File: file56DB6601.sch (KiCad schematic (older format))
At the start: 1 part, among them U2 SHT21

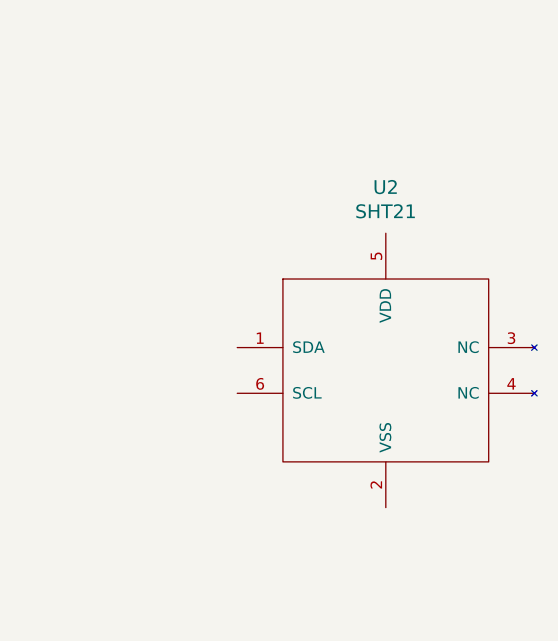
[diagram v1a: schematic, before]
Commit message: started layout, completed schematic
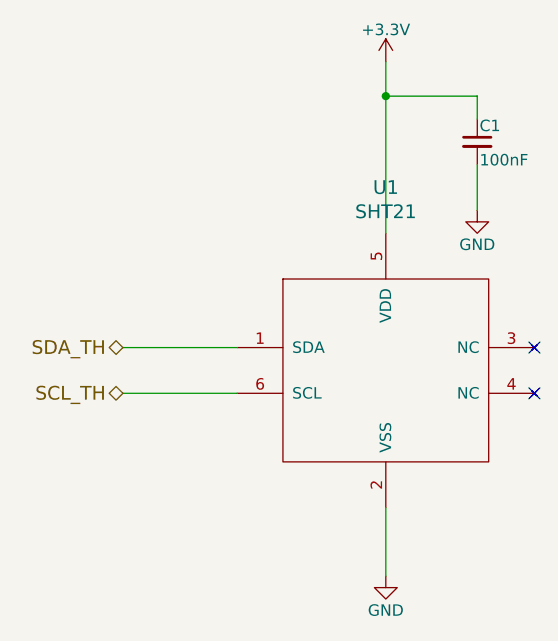
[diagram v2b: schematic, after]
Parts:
- added C1: 100nF, symbol C_Small
- renumbered U2 to U1
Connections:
- net SDA_TH: now reaches U1.1 (SDA)
- net GND: now reaches U1.2 (VSS)
- net GND: now also C1.2
- net +3V3: now reaches U1.5 (VDD)
- net +3V3: now also C1.1
- net SCL_TH: now reaches U1.6 (SCL)
- no-connect marks 0 -> 2
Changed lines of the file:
@@
 LIBS:mpu-9250
 LIBS:SAMD21E17A
+LIBS:miniultrapro
+LIBS:texas-instruments
 LIBS:lorawan_gps-cache
 EELAYER 25 0
@@
 $Descr A4 11693 8268
 encoding utf-8
-Sheet 3 7
+Sheet 2 7
 Title ""
 Date ""
@@
 $EndDescr
 $Comp
-L SHT21 U2
+L SHT21 U1
 U 1 1 56DB6717
 P 5650 3200
-F 0 "U2" H 5650 4000 60  0000 C CNN
+F 0 "U1" H 5650 4000 60  0000 C CNN
 F 1 "SHT21" H 5650 3894 60  0000 C CNN
 F 2 "timhawes:SHT21" H 5650 3200 60  0001 C CNN
@@
 	1    0    0    -1
 $EndComp
+$Comp
+L GND #PWR2
+U 1 1 56EA146B
+P 5650 4100
+F 0 "#PWR2" H 5650 3850 50  0001 C CNN
+F 1 "GND" H 5650 3950 50  0000 C CNN
+F 2 "" H 5650 4100 50  0000 C CNN
+F 3 "" H 5650 4100 50  0000 C CNN
+	1    5650 4100
+	1    0    0    -1
+$EndComp
+$Comp
+L +3.3V #PWR1
+U 1 1 56EA1481
+P 5650 1850
+F 0 "#PWR1" H 5650 1700 50  0001 C CNN
+F 1 "+3.3V" H 5650 1990 50  0000 C CNN
+F 2 "" H 5650 1850 50  0000 C CNN
+F 3 "" H 5650 1850 50  0000 C CNN
+	1    5650 1850
+	1    0    0    -1
+$EndComp
+$Comp
+L GND #PWR3
+U 1 1 56EA1497
+P 6050 2500
+F 0 "#PWR3" H 6050 2250 50  0001 C CNN
+F 1 "GND" H 6050 2350 50  0000 C CNN
+F 2 "" H 6050 2500 50  0000 C CNN
+F 3 "" H 6050 2500 50  0000 C CNN
+	1    6050 2500
+	1    0    0    -1
+$EndComp
+$Comp
+L C_Small C1
+U 1 1 56EA1572
+P 6050 2200
+F 0 "C1" H 6060 2270 50  0000 L CNN
+F 1 "100nF" H 6060 2120 50  0000 L CNN
+F 2 "" H 6050 2200 50  0000 C CNN
+F 3 "" H 6050 2200 50  0000 C CNN
+	1    6050 2200
+	1    0    0    -1
+$EndComp
+Wire Wire Line
+	5650 1850 5650 2600
+Wire Wire Line
+	6050 2100 6050 2000
+Wire Wire Line
+	6050 2000 5650 2000
+Connection ~ 5650 2000
+Wire Wire Line
+	6050 2300 6050 2500
+Wire Wire Line
+	5650 4100 5650 3800
+Text HLabel 4500 3100 0    60   BiDi ~ 0
+SDA_TH
+Text HLabel 4500 3300 0    60   BiDi ~ 0
+SCL_TH
+NoConn ~ 6300 3100
+NoConn ~ 6300 3300
+Wire Wire Line
+	4500 3100 5000 3100
+Wire Wire Line
+	4500 3300 5000 3300
 $EndSCHEMATC
